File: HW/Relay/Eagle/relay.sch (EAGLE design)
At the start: 48 parts, among them IC2 DS18B20, K2 CQ1-12V, M1 WIRELESS-NRF24L01, T1 BC847, U3 MCP16311, X1 MC3-G, X2 MC2-G, X3 MC2-G

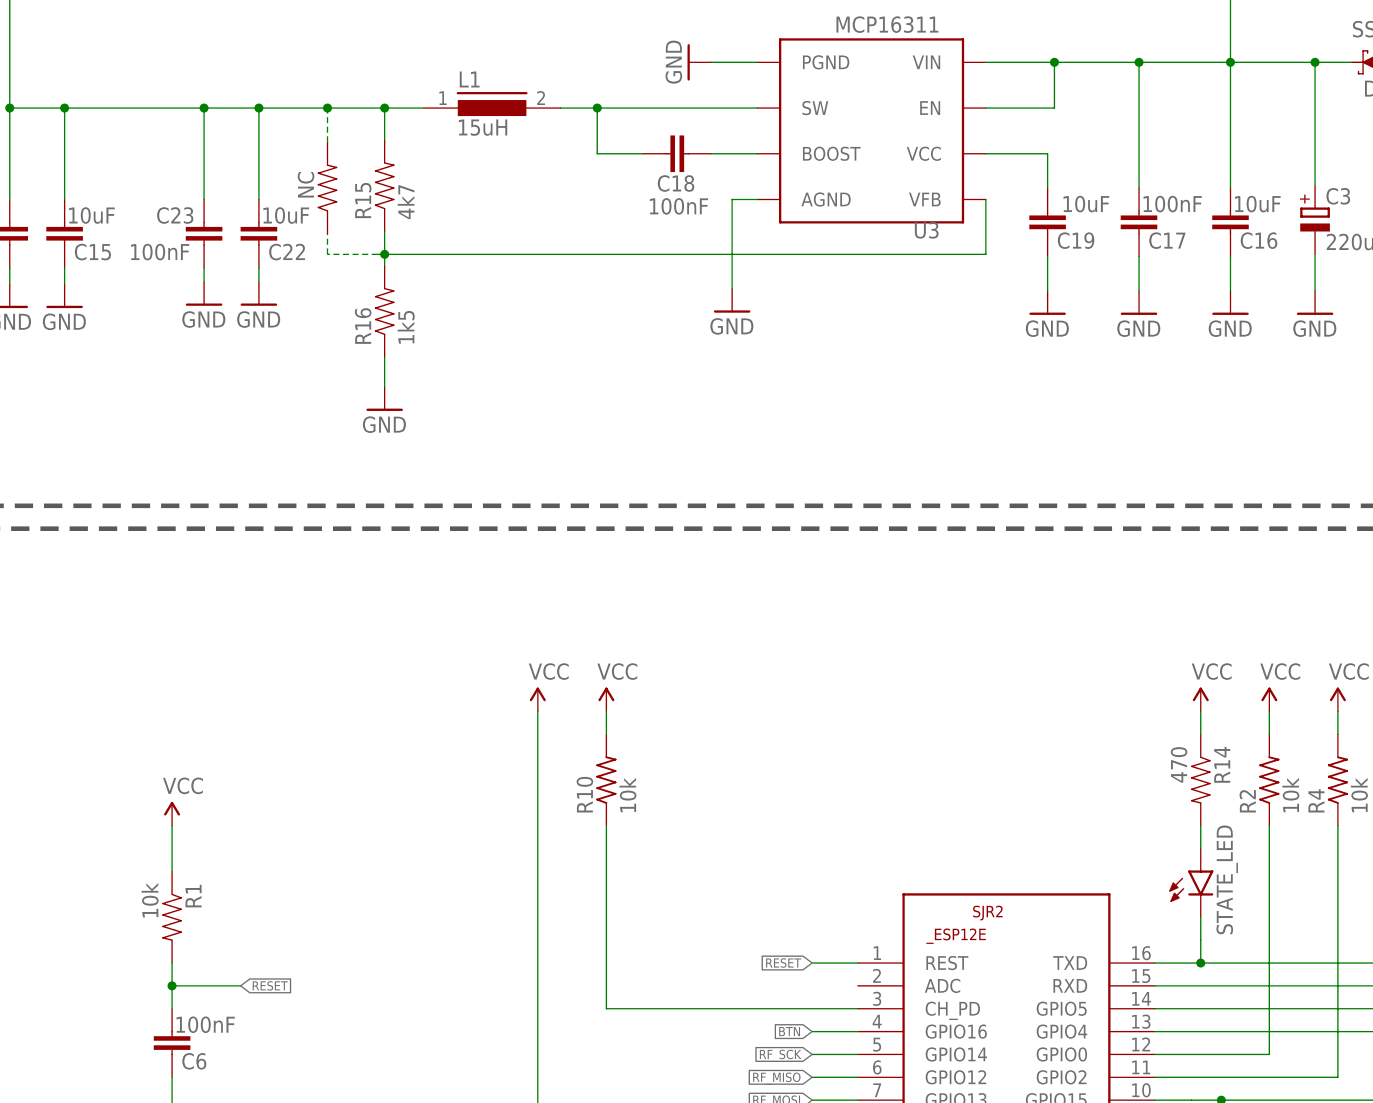
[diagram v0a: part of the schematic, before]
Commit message: Schematics are updated
Kickstart flasher PCB
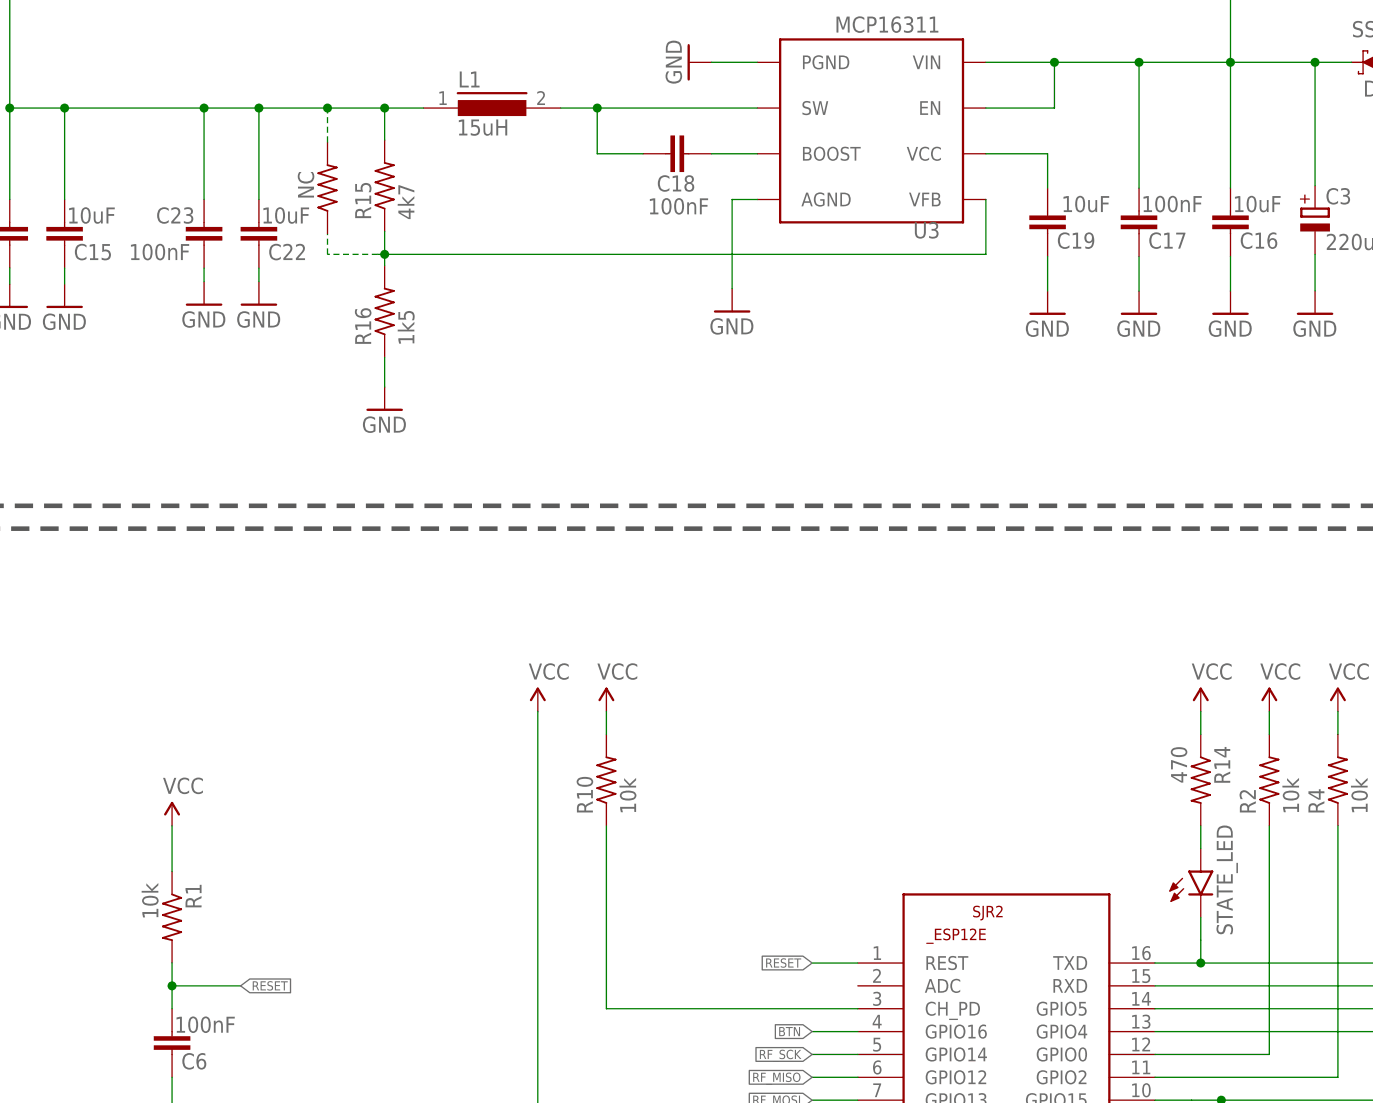
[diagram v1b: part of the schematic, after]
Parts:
- NC, R1, R14, R15, R16: device antduino:SPARKFUN_RESISTOR0805-RES -> rcl:R-US_M0805
- R10, R11, R12, R2, R3, R4, R5, R8, R9: device rcl:R-US_M2012 -> rcl:R-US_M0805
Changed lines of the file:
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@@
 <part name="GND33" library="supply1" deviceset="GND" device=""/>
 <part name="GND34" library="supply1" deviceset="GND" device=""/>
-<part name="R15" library="antduino" deviceset="SPARKFUN_RESISTOR" device="0805-RES" value="4k7"/>
-<part name="R16" library="antduino" deviceset="SPARKFUN_RESISTOR" device="0805-RES" value="1k5"/>
+<part name="R15" library="rcl" library_urn="urn:adsk.eagle:library:334" deviceset="R-US_" device="M0805" package3d_urn="urn:adsk.eagle:package:23556/2" value="4k7"/>
+<part name="R16" library="rcl" library_urn="urn:adsk.eagle:library:334" deviceset="R-US_" device="M0805" package3d_urn="urn:adsk.eagle:package:23556/2" value="1k5"/>
 <part name="GND35" library="supply1" deviceset="GND" device=""/>
-<part name="NC" library="antduino" deviceset="SPARKFUN_RESISTOR" device="0805-RES"/>
+<part name="NC" library="rcl" library_urn="urn:adsk.eagle:library:334" deviceset="R-US_" device="M0805" package3d_urn="urn:adsk.eagle:package:23556/2"/>
 <part name="SUPPLY11" library="SparkFun-Aesthetics" deviceset="VCC" device=""/>
 <part name="L1" library="inductors" library_urn="urn:adsk.eagle:library:243" deviceset="DR74" device="" package3d_urn="urn:adsk.eagle:package:15122/1" value="15uH"/>
@@
 <part name="C4" library="rcl" library_urn="urn:adsk.eagle:library:334" deviceset="C-EU" device="C0805" package3d_urn="urn:adsk.eagle:package:23617/2" value="100nF"/>
 <part name="C5" library="rcl" library_urn="urn:adsk.eagle:library:334" deviceset="C-EU" device="C0805" package3d_urn="urn:adsk.eagle:package:23617/2" value="10uF"/>
-<part name="R8" library="rcl" library_urn="urn:adsk.eagle:library:334" deviceset="R-US_" device="M2012" package3d_urn="urn:adsk.eagle:package:23561/2" value="1k"/>
-<part name="R9" library="rcl" library_urn="urn:adsk.eagle:library:334" deviceset="R-US_" device="M2012" package3d_urn="urn:adsk.eagle:package:23561/2" value="4k7"/>
-<part name="R10" library="rcl" library_urn="urn:adsk.eagle:library:334" deviceset="R-US_" device="M2012" package3d_urn="urn:adsk.eagle:package:23561/2" value="10k"/>
+<part name="R8" library="rcl" library_urn="urn:adsk.eagle:library:334" deviceset="R-US_" device="M0805" package3d_urn="urn:adsk.eagle:package:23556/2" value="1k"/>
+<part name="R9" library="rcl" library_urn="urn:adsk.eagle:library:334" deviceset="R-US_" device="M0805" package3d_urn="urn:adsk.eagle:package:23556/2" value="4k7"/>
+<part name="R10" library="rcl" library_urn="urn:adsk.eagle:library:334" deviceset="R-US_" device="M0805" package3d_urn="urn:adsk.eagle:package:23556/2" value="10k"/>
 <part name="TP1" library="testpad" library_urn="urn:adsk.eagle:library:385" deviceset="TP" device="TP20SQ" package3d_urn="urn:adsk.eagle:package:27980/1"/>
 <part name="TP2" library="testpad" library_urn="urn:adsk.eagle:library:385" deviceset="TP" device="TP20SQ" package3d_urn="urn:adsk.eagle:package:27980/1"/>
@@
 <part name="TP5" library="testpad" library_urn="urn:adsk.eagle:library:385" deviceset="TP" device="TP20SQ" package3d_urn="urn:adsk.eagle:package:27980/1"/>
 <part name="TP6" library="testpad" library_urn="urn:adsk.eagle:library:385" deviceset="TP" device="TP20SQ" package3d_urn="urn:adsk.eagle:package:27980/1"/>
-<part name="R1" library="antduino" deviceset="SPARKFUN_RESISTOR" device="0805-RES" value="10k"/>
+<part name="R1" library="rcl" library_urn="urn:adsk.eagle:library:334" deviceset="R-US_" device="M0805" package3d_urn="urn:adsk.eagle:package:23556/2" value="10k"/>
 <part name="C6" library="rcl" library_urn="urn:adsk.eagle:library:334" deviceset="C-EU" device="C0805" package3d_urn="urn:adsk.eagle:package:23617/2" value="100nF"/>
 <part name="GND3" library="supply1" deviceset="GND" device=""/>
 <part name="SUPPLY13" library="SparkFun-Aesthetics" deviceset="VCC" device=""/>
-<part name="R14" library="antduino" deviceset="SPARKFUN_RESISTOR" device="0805-RES" value="470"/>
+<part name="R14" library="rcl" library_urn="urn:adsk.eagle:library:334" deviceset="R-US_" device="M0805" package3d_urn="urn:adsk.eagle:package:23556/2" value="470"/>
 <part name="SUPPLY9" library="SparkFun-Aesthetics" deviceset="VCC" device=""/>
 <part name="STATE_LED" library="led" library_urn="urn:adsk.eagle:library:259" deviceset="LED" device="3MM" package3d_urn="urn:adsk.eagle:package:15797/1"/>
-<part name="R5" library="rcl" library_urn="urn:adsk.eagle:library:334" deviceset="R-US_" device="M2012" package3d_urn="urn:adsk.eagle:package:23561/2" value="4.7K"/>
-<part name="R11" library="rcl" library_urn="urn:adsk.eagle:library:334" deviceset="R-US_" device="M2012" package3d_urn="urn:adsk.eagle:package:23561/2" value="4.7K"/>
+<part name="R5" library="rcl" library_urn="urn:adsk.eagle:library:334" deviceset="R-US_" device="M0805" package3d_urn="urn:adsk.eagle:package:23556/2" value="4.7K"/>
+<part name="R11" library="rcl" library_urn="urn:adsk.eagle:library:334" deviceset="R-US_" device="M0805" package3d_urn="urn:adsk.eagle:package:23556/2" value="4.7K"/>
 <part name="GND5" library="supply1" library_urn="urn:adsk.eagle:library:371" deviceset="GND" device=""/>
-<part name="R12" library="rcl" library_urn="urn:adsk.eagle:library:334" deviceset="R-US_" device="M2012" package3d_urn="urn:adsk.eagle:package:23561/2" value="10k"/>
+<part name="R12" library="rcl" library_urn="urn:adsk.eagle:library:334" deviceset="R-US_" device="M0805" package3d_urn="urn:adsk.eagle:package:23556/2" value="10k"/>
 <part name="FRAME1" library="frames" library_urn="urn:adsk.eagle:library:229" deviceset="FRAME_B_L" device=""/>
 <part name="M1" library="diy-modules" deviceset="WIRELESS-NRF24L01" device=""/>
@@
 <part name="X2" library="con-phoenix-381_l" deviceset="MC2-G" device=""/>
 <part name="X3" library="con-phoenix-381_l" deviceset="MC2-G" device=""/>
-<part name="R2" library="rcl" library_urn="urn:adsk.eagle:library:334" deviceset="R-US_" device="M2012" package3d_urn="urn:adsk.eagle:package:23561/2" value="10k"/>
+<part name="R2" library="rcl" library_urn="urn:adsk.eagle:library:334" deviceset="R-US_" device="M0805" package3d_urn="urn:adsk.eagle:package:23556/2" value="10k"/>
 <part name="SUPPLY2" library="SparkFun-Aesthetics" deviceset="VCC" device=""/>
 <part name="GND10" library="supply1" library_urn="urn:adsk.eagle:library:371" deviceset="GND" device=""/>
-<part name="R3" library="rcl" library_urn="urn:adsk.eagle:library:334" deviceset="R-US_" device="M2012" package3d_urn="urn:adsk.eagle:package:23561/2" value="10K"/>
+<part name="R3" library="rcl" library_urn="urn:adsk.eagle:library:334" deviceset="R-US_" device="M0805" package3d_urn="urn:adsk.eagle:package:23556/2" value="10K"/>
 <part name="SUPPLY1" library="SparkFun-Aesthetics" deviceset="VCC" device=""/>
 <part name="SUPPLY3" library="SparkFun-Aesthetics" deviceset="VCC" device=""/>
@@
 <part name="SUPPLY5" library="SparkFun-Aesthetics" deviceset="VCC" device=""/>
 <part name="SUPPLY6" library="SparkFun-Aesthetics" deviceset="VCC" device=""/>
-<part name="R4" library="rcl" library_urn="urn:adsk.eagle:library:334" deviceset="R-US_" device="M2012" package3d_urn="urn:adsk.eagle:package:23561/2" value="10k"/>
+<part name="R4" library="rcl" library_urn="urn:adsk.eagle:library:334" deviceset="R-US_" device="M0805" package3d_urn="urn:adsk.eagle:package:23556/2" value="10k"/>
 <part name="SUPPLY7" library="SparkFun-Aesthetics" deviceset="VCC" device=""/>
 <part name="C3" library="rcl" library_urn="urn:adsk.eagle:library:334" deviceset="CPOL-EU" device="150CLZ-0810" package3d_urn="urn:adsk.eagle:package:23394/2" value="220uF 35V"/>
